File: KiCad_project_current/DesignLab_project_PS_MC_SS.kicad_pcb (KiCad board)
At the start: 2 copper layers, 120.4 x 91.9 mm, 61 parts, among them J1 Conn_01x09, J2 USB_B_Micro, J3 Barrel_Jack, J4 Conn_02x08_Odd_Even, SW1 SW_Push, SW2 SW_Push, SW3 SW_Push, SW4 SW_Push, SW5 SW_Push, U1 ATmega328P-P, U2 CH340C, U3 BMP280, U4 DS18B20, U5 L7805, U6 LTC-4627JD, U7 LM1117DT-3.3, Y1 16MHz

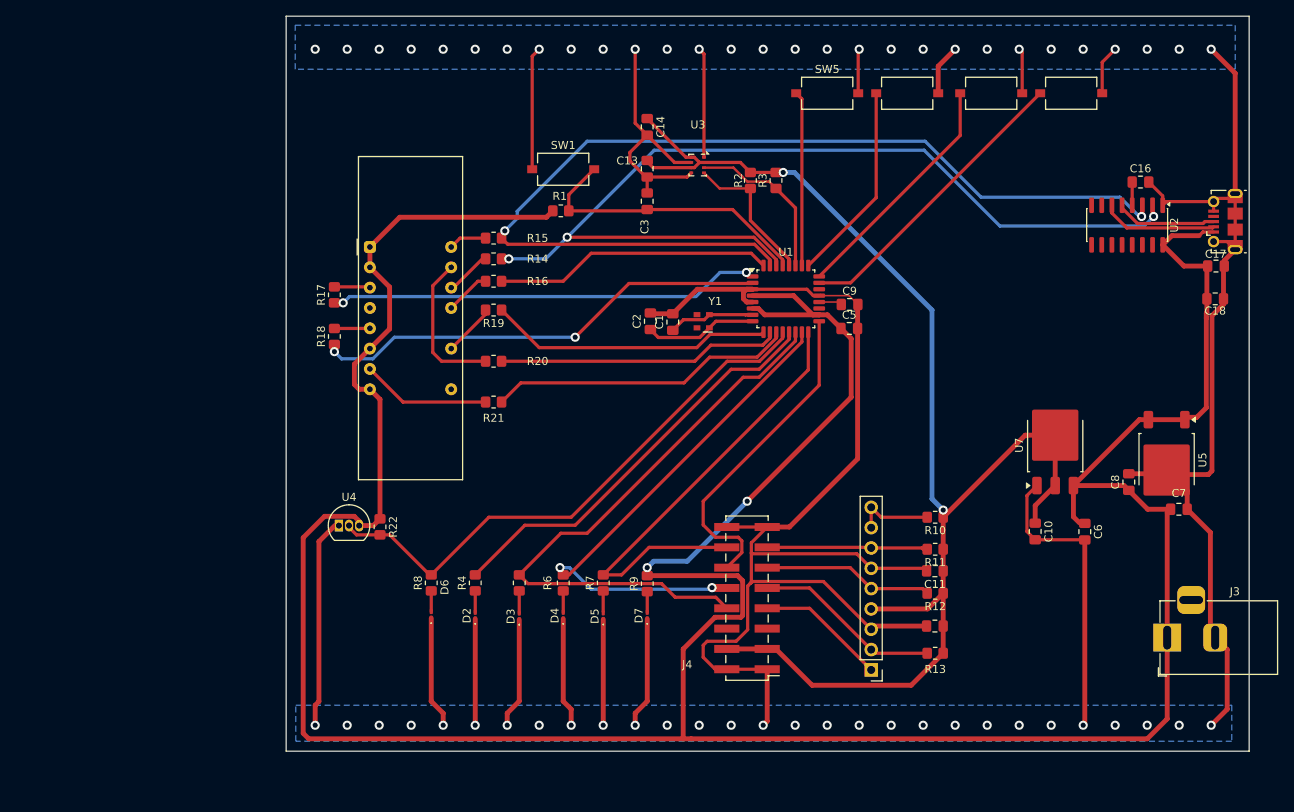
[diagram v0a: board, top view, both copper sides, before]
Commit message: Final version of the KiCad project
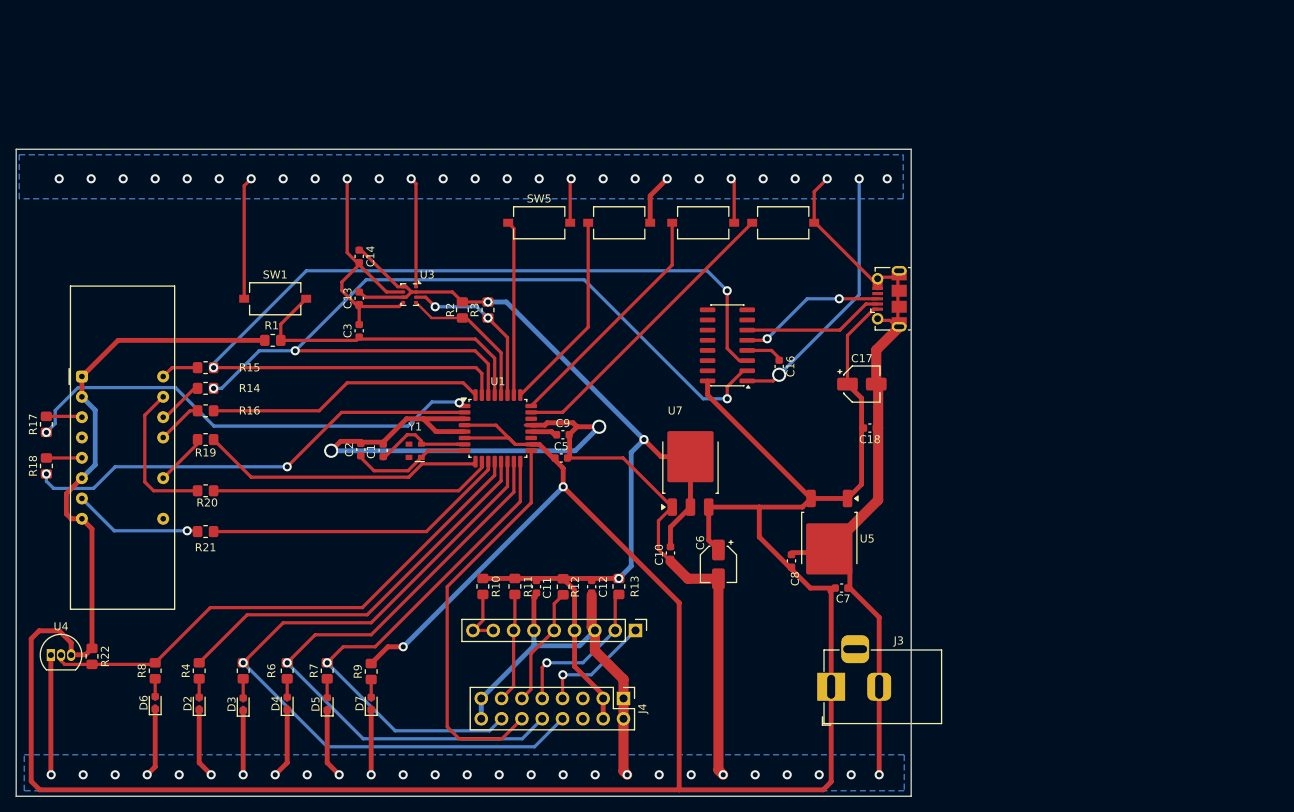
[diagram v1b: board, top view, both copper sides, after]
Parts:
- C1, C10, C11, C12, C13, C14, C16, C18, C2, C3, C5, C7, C8, C9: footprint Capacitor_SMD:C_0805_2012Metric_Pad1.18x1.45mm_HandSolder -> Capacitor_SMD:C_0603_1608Metric
- C17, C6: footprint Capacitor_SMD:C_0805_2012Metric_Pad1.18x1.45mm_HandSolder -> Capacitor_SMD:CP_Elec_4x3
- D2, D3, D4, D5, D6, D7: footprint LED_SMD:LED_0201_0603Metric_Pad0.64x0.40mm_HandSolder -> LED_SMD:LED_0603_1608Metric
- J4: footprint Connector_PinHeader_2.54mm:PinHeader_2x08_P2.54mm_Vertical_SMD -> Connector_PinHeader_2.54mm:PinHeader_2x08_P2.54mm_Vertical
- R4, R5, R6, R7, R8, R9: value 1kOhm -> 1k
- moved R10 57.2 mm to (148.5, 108.2), turned to -90 degrees
- moved R11 52.7 mm to (152.5, 108.2), turned to -90 degrees
- moved U2 52.2 mm to (179.0, 78.0), turned to 180 degrees
- moved C16 50.7 mm to (185.5, 80.7), turned to -90 degrees
- moved C11 49.8 mm to (155.2, 108.2), turned to -90 degrees
- moved C17 46.7 mm to (195.8, 82.9)
- moved R12 46.5 mm to (158.5, 108.2), turned to -90 degrees
- moved C18 46.1 mm to (196.8, 88.4)
- moved C6 46.0 mm to (177.9, 105.4)
- moved C10 45.7 mm to (171.9, 104.0)
- moved U7 45.7 mm to (174.4, 93.2)
- moved U5 43.3 mm to (191.8, 102.2)
- moved C7 43.3 mm to (193.3, 108.4)
- moved C8 43.3 mm to (187.0, 105.0)
- moved C12 43.2 mm to (162.1, 108.2), turned to -90 degrees
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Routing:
- net GND: track 511.6 -> 459.7 mm, vias 58 -> 57
- net +3.3V: track 165.3 -> 126.9 mm, vias 2 -> 3
- net PB2: track 75.4 -> 91.0 mm, vias 0 -> 1
- net PB3: track 63.3 -> 77.8 mm, vias 2 -> 1
- net RX/PD0: track 118.7 -> 109.5 mm
- net PB5: track 41.2 -> 49.8 mm
- net PD3: track 52.0 -> 59.0 mm
- net TX/PD1: track 124.0 -> 117.4 mm
- net MISO: track 20.1 -> 13.7 mm
- net SCK: track 21.3 -> 15.1 mm
- net PB4: track 57.9 -> 64.1 mm, vias 0 -> 1
- net D+: track 13.0 -> 18.7 mm, vias 0 -> 2
- net MOSI: track 23.4 -> 19.6 mm, vias 0 -> 1
- net +5V: track 408.6 -> 405.1 mm
- net D-: track 14.5 -> 17.7 mm
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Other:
- board size 120.4 x 91.9 mm -> 111.9 x 80.9 mm
